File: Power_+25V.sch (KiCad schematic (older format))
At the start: 14 parts

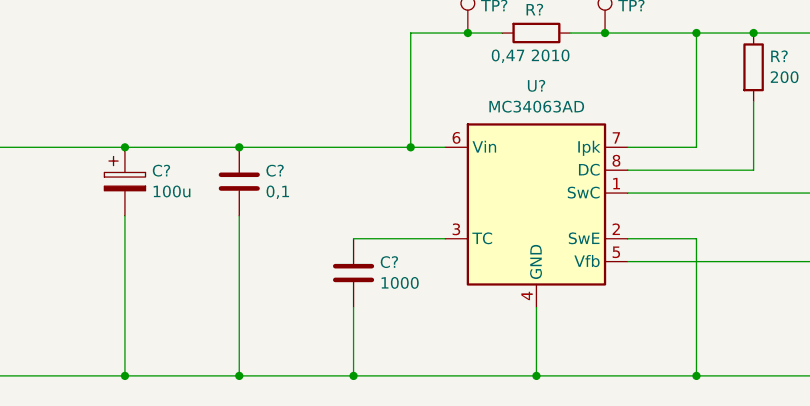
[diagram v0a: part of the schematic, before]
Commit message: Add files via upload
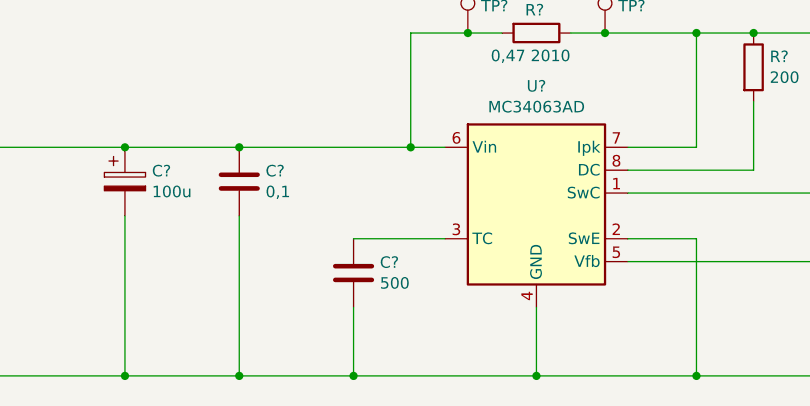
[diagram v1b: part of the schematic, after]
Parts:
- C?: value 1000 -> 500
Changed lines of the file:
@@
 AR Path="/60DF0860/60E81588" Ref="C?"  Part="1"
 F 0 "C?" H 4615 4596 50  0000 L CNN
-F 1 "1000" H 4615 4505 50  0000 L CNN
+F 1 "500" H 4615 4505 50  0000 L CNN
 F 2 "Capacitor_SMD:C_0603_1608Metric_Pad1.08x0.95mm_HandSolder" H 4538 4400 50  0001 C CNN
 F 3 "~" H 4500 4550 50  0001 C CNN

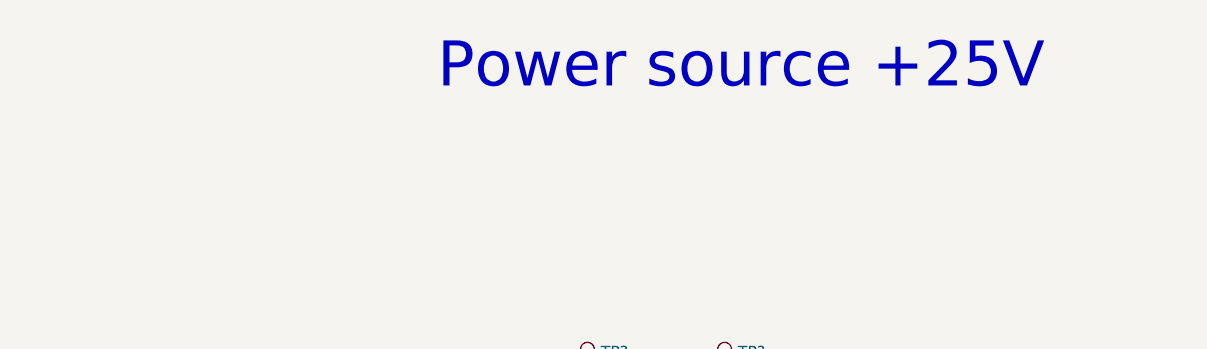
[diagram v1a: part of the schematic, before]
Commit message: Add files via upload
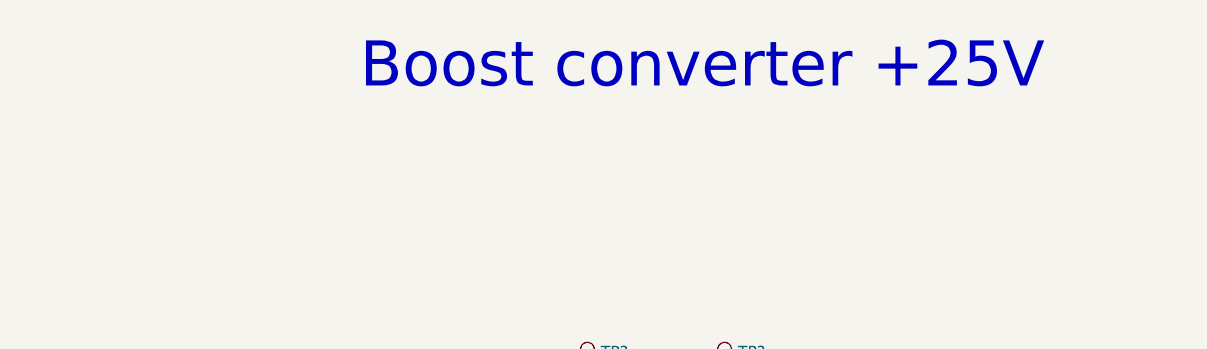
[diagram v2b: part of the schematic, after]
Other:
- note added: "Boost converter +25V"
- note removed: "Power source +25V"
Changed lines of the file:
@@
 $Descr A4 11693 8268
 encoding utf-8
-Sheet 7 15
+Sheet 7 20
 Title ""
 Date ""
@@
 $EndDescr
 Text Notes 7000 2250 2    197  ~ 0
-Power source +25V
+Boost converter +25V
 $Comp
 L Device:C C?

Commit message: Add files via upload
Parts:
- removed C?: 100u, symbol Device:CP
- removed TP?: TestPoint, symbol Connector:TestPoint
- added C?: 100u, symbol Device:CP
- added TP?: TestPoint, symbol Connector:TestPoint
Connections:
- net +5V_IN: now also C?.1
- net GND: now also C?.2
- net at L?.1, R?.1, R?.1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: now also TP?.1
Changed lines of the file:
@@
 $Descr A4 11693 8268
 encoding utf-8
-Sheet 7 20
+Sheet 7 24
 Title ""
 Date ""
@@
 $Comp
 L Connector:TestPoint TP?
-U 1 1 60ACAEBE
+U 1 1 60F5917B
 P 5600 3500
-AR Path="/60ACAEBE" Ref="TP?"  Part="1"
-AR Path="/609FED99/60ACAEBE" Ref="TP?"  Part="1"
-AR Path="/60DF0860/60ACAEBE" Ref="TP?"  Part="1"
+AR Path="/60F5917B" Ref="TP?"  Part="1"
+AR Path="/609FED99/60F5917B" Ref="TP?"  Part="1"
+AR Path="/60DF0860/60F5917B" Ref="TP?"  Part="1"
 F 0 "TP?" H 5658 3618 50  0000 L CNN
 F 1 "TestPoint" H 5658 3527 50  0001 L CNN
@@
 $Comp
 L Device:CP C?
-U 1 1 60ADA476
+U 1 1 60F5917D
 P 3500 4150
 F 0 "C?" H 3618 4196 50  0000 L CNN
